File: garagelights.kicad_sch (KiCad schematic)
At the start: 40 parts, among them J1 Samtec SSW-104-03-F-S-RA, J2 Samtec SSW-106-01-L-S, J3 Screw_Terminal_01x01, J4 Screw_Terminal_01x01, Q1 ZVN4206AV, Q2 ZVN4206AV, Q3 ZVN4206AV, U1 NE555P, U2 NE555P, U3 4013, U4 LM7805_TO220, U5 4013

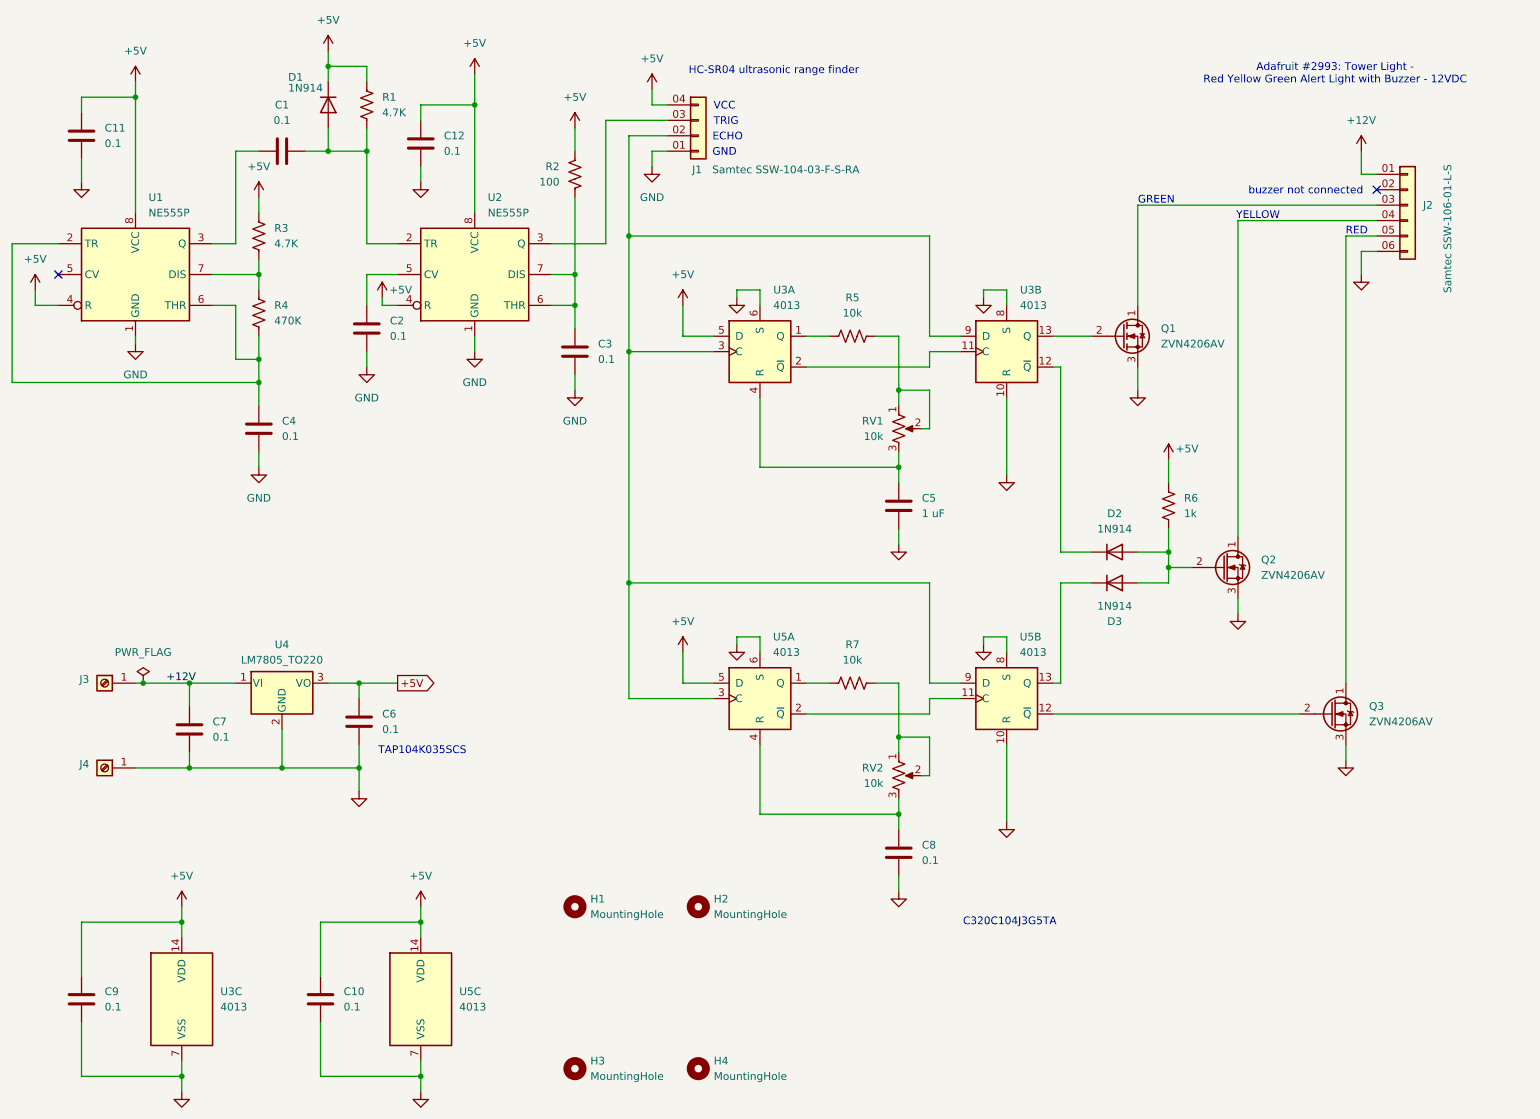
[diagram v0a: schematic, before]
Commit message: Rev A: as submitted to Osh Park order #fmnAZ4b4
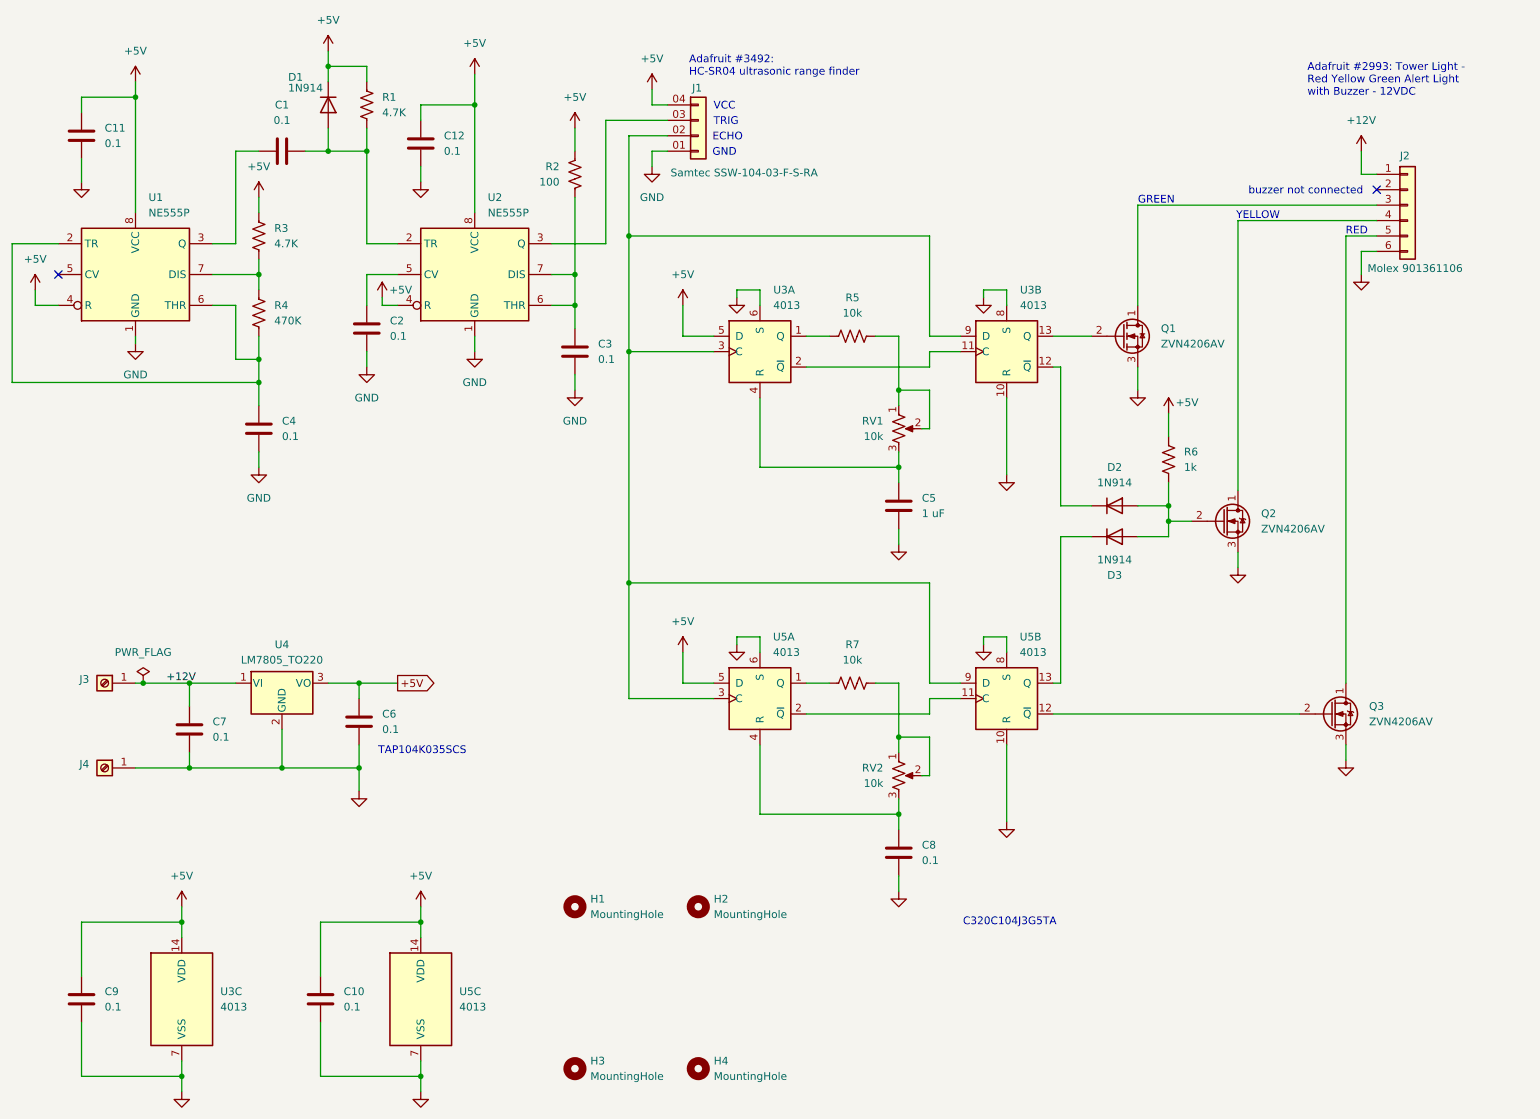
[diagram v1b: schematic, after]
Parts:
- J2: value Samtec SSW-106-01-L-S -> Molex 901361106; footprint Library:SAMTEC_SSW-106-01-X-S -> Library:CONN_SDA-90136_V_06_MOL
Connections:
- net +12V: now also J2.1 (Pin_1); no longer J2.01 (Pin_1)
- net GND: now also J2.6 (Pin_6); no longer J2.06 (Pin_6)
- net at Q3.1 (D): now also J2.5 (Pin_5); no longer J2.05 (Pin_5)
- net at Q2.1 (D): now also J2.4 (Pin_4); no longer J2.04 (Pin_4)
- net at Q1.1 (D): now also J2.3 (Pin_3); no longer J2.03 (Pin_3)
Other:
- note added: "Adafruit #3492: HC-SR04 ultrasonic range finder"
- note removed: "HC-SR04 ultrasonic range finder"
- title: (none) -> Garage Lights
- moved on the sheet: D2, D3, Q2, R6
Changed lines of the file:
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@@
 	(generator_version "9.0")
 	(paper "USLetter")
-	(text "HC-SR04 ultrasonic range finder"
+	(title_block
+		(title "Garage Lights")
+		(rev "A")
+		(comment 4 "Firmware-free ultrasonic range finder")
+	)
+	(text "Adafruit #3492:\nHC-SR04 ultrasonic range finder"
 		(exclude_from_sim no)
-		(at 148.336 24.892 0)
+		(at 134.366 24.13 0)
 		(effects
 			(font
 				(size 1.27 1.27)
 			)
+			(justify left)
 		)
 	)
@@
 		)
 	)
-	(text "Adafruit #2993: Tower Light - \nRed Yellow Green Alert Light with Buzzer - 12VDC"
+	(text "Adafruit #2993: Tower Light - \nRed Yellow Green Alert Light\nwith Buzzer - 12VDC"
 		(exclude_from_sim no)
-		(at 240.792 25.4 0)
+		(at 236.22 26.416 0)
 		(effects
 			(font
 				(size 1.27 1.27)
 			)
+			(justify left)
 		)
 	)
@@
 	)
 	(junction
-		(at 213.36 104.14)
+		(at 213.36 96.52)
 		(diameter 0)
 		(color 0 0 0 0)
@@
 	)
 	(junction
-		(at 213.36 106.68)
+		(at 213.36 99.06)
 		(diameter 0)
 		(color 0 0 0 0)
@@
 	(wire
 		(pts
-			(xy 213.36 106.68) (xy 217.17 106.68)
+			(xy 213.36 99.06) (xy 217.17 99.06)
 		)
 		(stroke
@@
 	(wire
 		(pts
-			(xy 213.36 106.68) (xy 213.36 109.22)
+			(xy 213.36 99.06) (xy 213.36 101.6)
 		)
 		(stroke
@@
 	(wire
 		(pts
-			(xy 195.58 73.66) (xy 195.58 104.14)
+			(xy 195.58 73.66) (xy 195.58 96.52)
 		)
 		(stroke
@@
 	(wire
 		(pts
-			(xy 224.79 111.76) (xy 224.79 114.3)
+			(xy 224.79 104.14) (xy 224.79 106.68)
 		)
 		(stroke
@@
 	(wire
 		(pts
-			(xy 195.58 104.14) (xy 200.66 104.14)
+			(xy 195.58 96.52) (xy 200.66 96.52)
 		)
 		(stroke
@@
 	(wire
 		(pts
-			(xy 213.36 104.14) (xy 213.36 106.68)
+			(xy 213.36 96.52) (xy 213.36 99.06)
 		)
 		(stroke
@@
 	(wire
 		(pts
-			(xy 208.28 109.22) (xy 213.36 109.22)
+			(xy 208.28 101.6) (xy 213.36 101.6)
 		)
 		(stroke
@@
 	(wire
 		(pts
-			(xy 224.79 49.53) (xy 224.79 101.6)
+			(xy 224.79 49.53) (xy 224.79 93.98)
 		)
 		(stroke
@@
 	(wire
 		(pts
-			(xy 195.58 109.22) (xy 200.66 109.22)
+			(xy 195.58 101.6) (xy 200.66 101.6)
 		)
 		(stroke
@@
 	(wire
 		(pts
-			(xy 213.36 88.9) (xy 213.36 92.71)
+			(xy 213.36 81.28) (xy 213.36 85.09)
 		)
 		(stroke
@@
 	(wire
 		(pts
-			(xy 208.28 104.14) (xy 213.36 104.14)
+			(xy 208.28 96.52) (xy 213.36 96.52)
 		)
 		(stroke
@@
 	(wire
 		(pts
-			(xy 195.58 125.73) (xy 195.58 109.22)
+			(xy 195.58 125.73) (xy 195.58 101.6)
 		)
 		(stroke
@@
 	(wire
 		(pts
-			(xy 213.36 100.33) (xy 213.36 104.14)
+			(xy 213.36 92.71) (xy 213.36 96.52)
 		)
 		(stroke
@@
 	(symbol
 		(lib_id "power:+5V")
-		(at 213.36 88.9 0)
+		(at 213.36 81.28 0)
 		(unit 1)
 		(exclude_from_sim no)
@@
 		(dnp no)
 		(property "Reference" "#PWR020"
-			(at 213.36 92.71 0)
+			(at 213.36 85.09 0)
 			(effects
 				(font
@@
 		)
 		(property "Value" "+5V"
-			(at 216.408 87.122 0)
+			(at 216.408 79.502 0)
 			(effects
 				(font
@@
 		)
 		(property "Footprint" ""
-			(at 213.36 88.9 0)
+			(at 213.36 81.28 0)
 			(effects
 				(font
@@
 		)
 		(property "Datasheet" ""
-			(at 213.36 88.9 0)
+			(at 213.36 81.28 0)
 			(effects
 				(font
@@
 		)
 		(property "Description" "Power symbol creates a global label with name \"+5V\""
-			(at 213.36 88.9 0)
+			(at 213.36 81.28 0)
 			(effects
 				(font
@@
 	(symbol
 		(lib_id "Diode:1N914")
-		(at 204.47 109.22 0)
+		(at 204.47 101.6 0)
 		(mirror x)
 		(unit 1)
@@
 		(dnp no)
 		(property "Reference" "D3"
-			(at 204.47 115.57 0)
+			(at 204.47 107.95 0)
 			(effects
 				(font
@@
 		)
 		(property "Value" "1N914"
-			(at 204.47 113.03 0)
+			(at 204.47 105.41 0)
 			(effects
 				(font
@@
 		)
 		(property "Footprint" "Diode_THT:D_DO-35_SOD27_P7.62mm_Horizontal"
-			(at 204.47 104.775 0)
+			(at 204.47 97.155 0)
 			(effects
 				(font
@@
 		)
 		(property "Datasheet" "http://www.vishay.com/docs/85622/1n914.pdf"
-			(at 204.47 109.22 0)
+			(at 204.47 101.6 0)
 			(effects
 				(font
@@
 		)
 		(property "Description" "100V 0.3A Small Signal Fast Switching Diode, DO-35"
-			(at 204.47 109.22 0)
+			(at 204.47 101.6 0)
 			(effects
 				(font
@@
 		)
 		(property "Sim.Device" "D"
-			(at 204.47 109.22 0)
+			(at 204.47 101.6 0)
 			(effects
 				(font
@@
 		)
 		(property "Sim.Pins" "1=K 2=A"
-			(at 204.47 109.22 0)
+			(at 204.47 101.6 0)
 			(effects
 				(font
@@
 	(symbol
 		(lib_id "Transistor_FET_Other:Q_NMOS_Depletion_DGS")
-		(at 222.25 106.68 0)
+		(at 222.25 99.06 0)
 		(unit 1)
 		(exclude_from_sim no)
@@
 		(fields_autoplaced yes)
 		(property "Reference" "Q2"
-			(at 228.6 105.4099 0)
+			(at 228.6 97.7899 0)
 			(effects
 				(font
@@
 		)
 		(property "Value" "ZVN4206AV"
-			(at 228.6 107.9499 0)
+			(at 228.6 100.3299 0)
 			(effects
 				(font
@@
 		)
 		(property "Footprint" "Package_TO_SOT_THT:TO-92S"
-			(at 222.25 106.68 0)
+			(at 222.25 99.06 0)
 			(effects
 				(font
@@
 		)
 		(property "Datasheet" "~"
-			(at 222.25 106.68 0)
+			(at 222.25 99.06 0)
 			(effects
 				(font
@@
 		)
 		(property "Description" "Depletion-mode N-channel MOSFET, drain/gate/source"
-			(at 222.25 106.68 0)
+			(at 222.25 99.06 0)
 			(effects
 				(font
@@
 	(symbol
 		(lib_id "Device:R_US")
-		(at 213.36 96.52 0)
+		(at 213.36 88.9 0)
 		(unit 1)
 		(exclude_from_sim no)
@@
 		(fields_autoplaced yes)
 		(property "Reference" "R6"
-			(at 215.9 95.2499 0)
+			(at 215.9 87.6299 0)
 			(effects
 				(font
@@
 		)
 		(property "Value" "1k"
-			(at 215.9 97.7899 0)
+			(at 215.9 90.1699 0)
 			(effects
 				(font
@@
 		)
 		(property "Footprint" "Resistor_THT:R_Axial_DIN0204_L3.6mm_D1.6mm_P7.62mm_Horizontal"
-			(at 214.376 96.774 90)
+			(at 214.376 89.154 90)
 			(effects
 				(font
@@
 		)
 		(property "Datasheet" "~"
-			(at 213.36 96.52 0)
+			(at 213.36 88.9 0)
 			(effects
 				(font
@@
 		)
 		(property "Description" "Resistor, US symbol"
-			(at 213.36 96.52 0)
+			(at 213.36 88.9 0)
 			(effects
 				(font
@@
 	(symbol
 		(lib_id "power:GND")
-		(at 224.79 114.3 0)
+		(at 224.79 106.68 0)
 		(unit 1)
 		(exclude_from_sim no)
@@
 		(fields_autoplaced yes)
 		(property "Reference" "#PWR024"
-			(at 224.79 120.65 0)
+			(at 224.79 113.03 0)
 			(effects
 				(font
@@
 		)
 		(property "Value" "GND"
-			(at 224.79 119.38 0)
+			(at 224.79 111.76 0)
 			(effects
 				(font
@@
 		)
 		(property "Footprint" ""
-			(at 224.79 114.3 0)
+			(at 224.79 106.68 0)
 			(effects
 				(font
@@
 		)
 		(property "Datasheet" ""
-			(at 224.79 114.3 0)
+			(at 224.79 106.68 0)
 			(effects
 				(font
@@
 		)
 		(property "Description" "Power symbol creates a global label with name \"GND\" , ground"
-			(at 224.79 114.3 0)
+			(at 224.79 106.68 0)
 			(effects
 				(font
@@
 		(dnp no)
 		(property "Reference" "J1"
-			(at 134.874 41.148 0)
+			(at 134.874 27.686 0)
 			(effects
 				(font
@@
 		)
 		(property "Value" "Samtec SSW-104-03-F-S-RA"
-			(at 138.176 41.148 0)
+			(at 131.318 41.656 0)
 			(effects
 				(font
@@
 		(dnp no)
 		(property "Reference" "J2"
-			(at 255.27 46.9899 0)
+			(at 251.46 38.862 0)
 			(effects
 				(font
@@
 			)
 		)
-		(property "Value" "Samtec SSW-106-01-L-S"
-			(at 259.334 61.468 90)
+		(property "Value" "Molex 901361106"
+			(at 246.126 57.404 0)
 			(effects
 				(font
@@
 			)
 		)
-		(property "Footprint" "Library:SAMTEC_SSW-106-01-X-S"
+		(property "Footprint" "Library:CONN_SDA-90136_V_06_MOL"
 			(at 252.73 46.99 0)
 			(effects
@@
 			)
 		)
-		(pin "05"
+		(pin "4"
 		)
-		(pin "02"
+		(pin "1"
 		)
-		(pin "06"
+		(pin "5"
 		)
-		(pin "04"
+		(pin "3"
 		)
-		(pin "03"
+		(pin "2"
 		)
-		(pin "01"
+		(pin "6"
 		)
 		(instances
@@
 	(symbol
 		(lib_id "Diode:1N914")
-		(at 204.47 104.14 0)
+		(at 204.47 96.52 0)
 		(unit 1)
 		(exclude_from_sim no)
@@
 		(dnp no)
 		(property "Reference" "D2"
-			(at 204.47 97.79 0)
+			(at 204.47 90.17 0)
 			(effects
 				(font
@@
 		)
 		(property "Value" "1N914"
-			(at 204.47 100.33 0)
+			(at 204.47 92.71 0)
 			(effects
 				(font
@@
 		)
 		(property "Footprint" "Diode_THT:D_DO-35_SOD27_P7.62mm_Horizontal"
-			(at 204.47 108.585 0)
+			(at 204.47 100.965 0)
 			(effects
 				(font
@@
 		)
 		(property "Datasheet" "http://www.vishay.com/docs/85622/1n914.pdf"
-			(at 204.47 104.14 0)
+			(at 204.47 96.52 0)
 			(effects
 				(font
@@
 		)
 		(property "Description" "100V 0.3A Small Signal Fast Switching Diode, DO-35"
-			(at 204.47 104.14 0)
+			(at 204.47 96.52 0)
 			(effects
 				(font
@@
 		)
 		(property "Sim.Device" "D"
-			(at 204.47 104.14 0)
+			(at 204.47 96.52 0)
 			(effects
 				(font
@@
 		)
 		(property "Sim.Pins" "1=K 2=A"
-			(at 204.47 104.14 0)
+			(at 204.47 96.52 0)
 			(effects
 				(font
